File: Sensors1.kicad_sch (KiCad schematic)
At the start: 12 parts, among them U26 BNO085

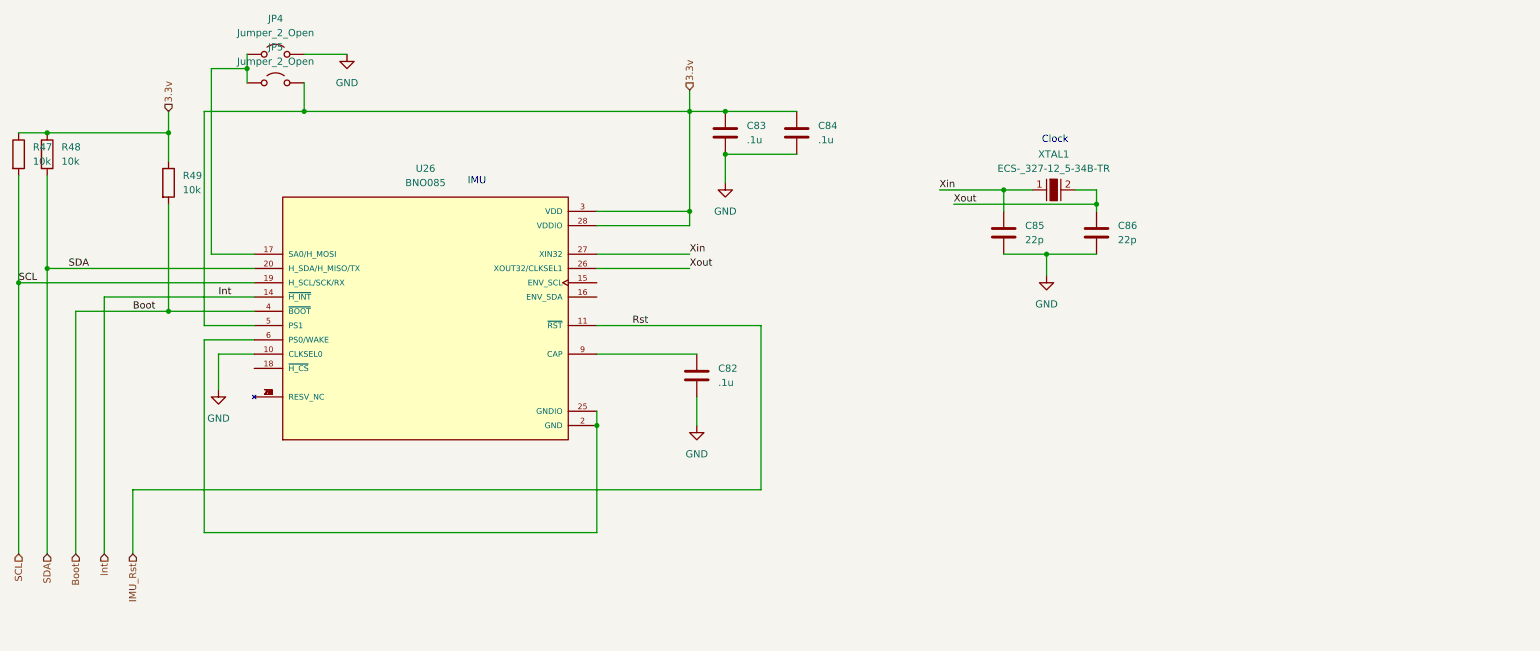
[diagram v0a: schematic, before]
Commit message: stuff
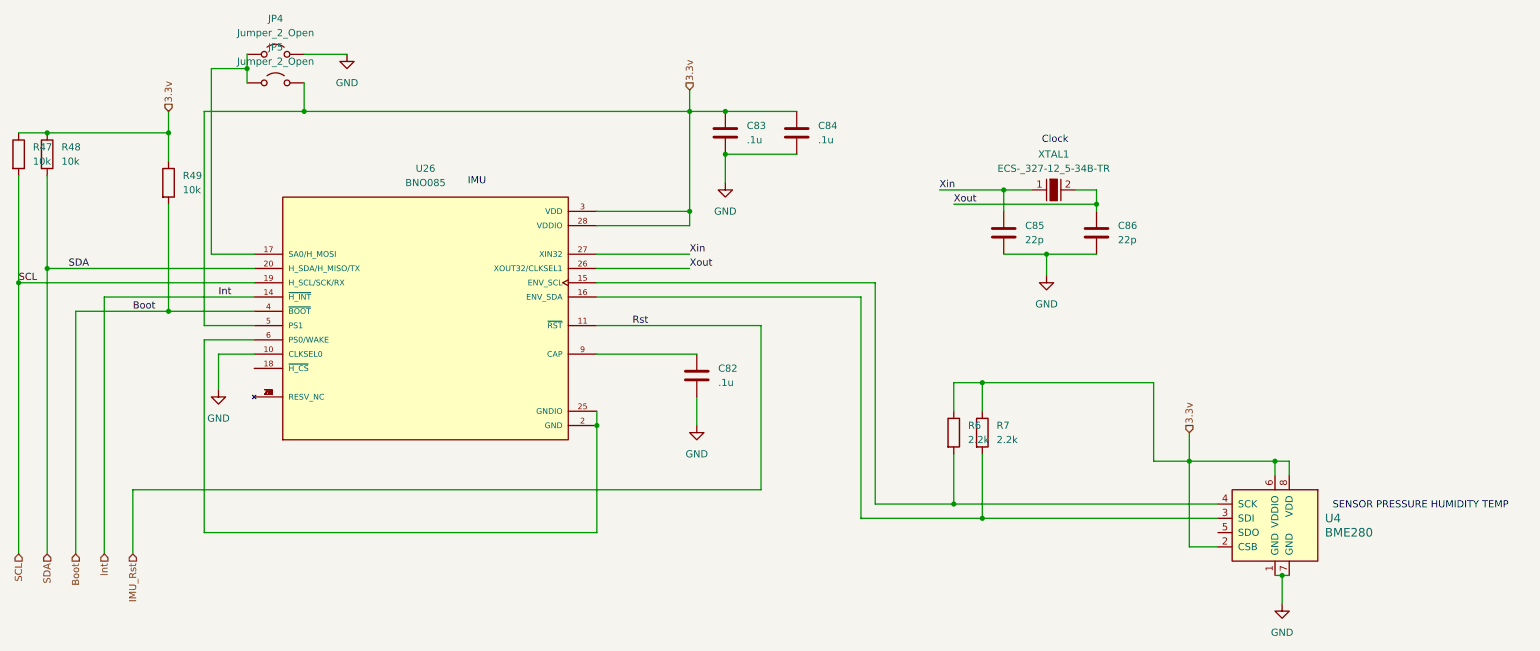
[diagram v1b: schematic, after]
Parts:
- added R6, R7: 2.2k, symbol Device:R
- added U4: BME280, digikey-footprints:Pressure_Sensor_LGA-8_2.5x2.5mm_BME280, symbol dk_Humidity-Moisture-Sensors:BME280
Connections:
- net 3.3v: now also R6.1, R7.1, U4.2 (CSB), U4.6 (VDDIO), U4.8 (VDD)
- net GND: now also U4.1 (GND), U4.7 (GND)
- net at U26.15 (ENV_SCL): now also R6.2, U4.4 (SCK)
- net at U26.16 (ENV_SDA): now also R7.2, U4.3 (SDI)
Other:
- note added: "SENSOR PRESSURE HUMIDITY TEMP"
